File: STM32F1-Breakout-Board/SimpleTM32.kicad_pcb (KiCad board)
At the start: 2 copper layers, 41 x 36 mm, 26 parts, among them J1 USB_B_Micro, J2 Conn_01x15, J3 Conn_01x15, U1 XC6206P332MR, U2 STM32F103C8T6, Y1 8MHz

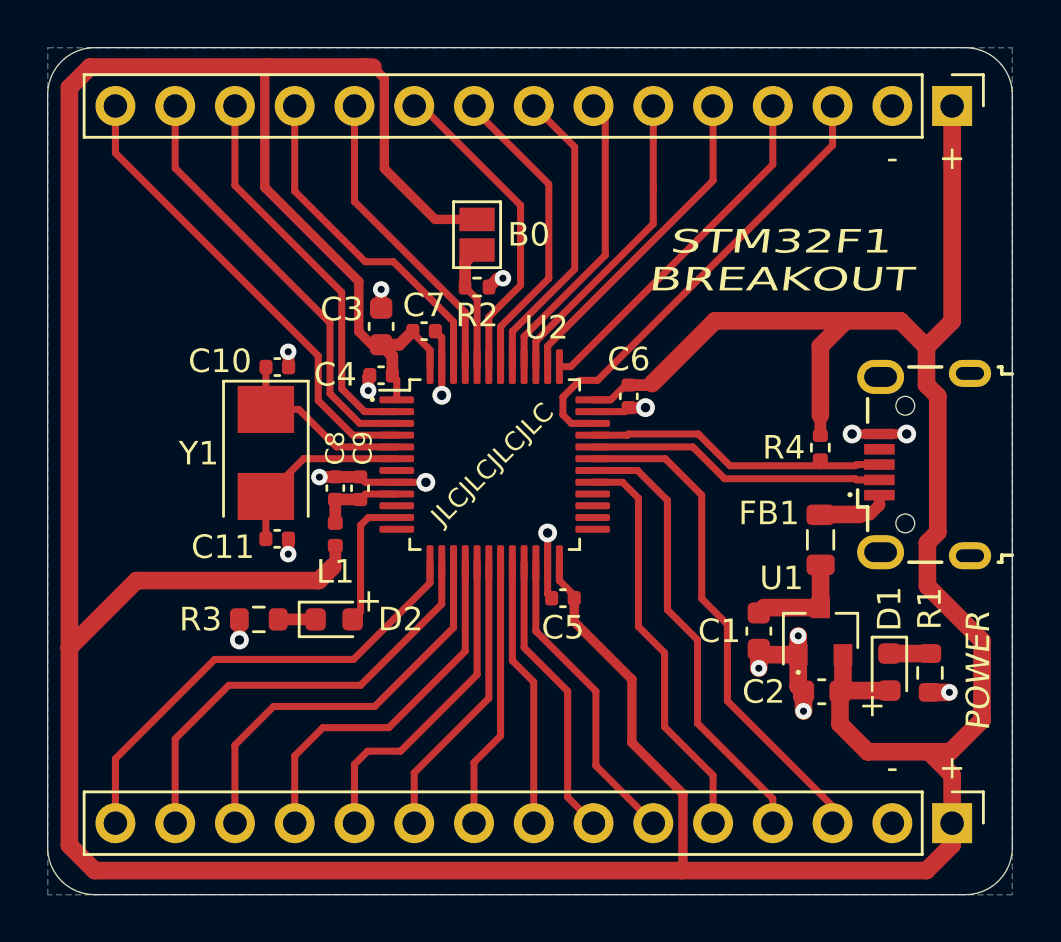
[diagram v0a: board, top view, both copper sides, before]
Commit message: rasp
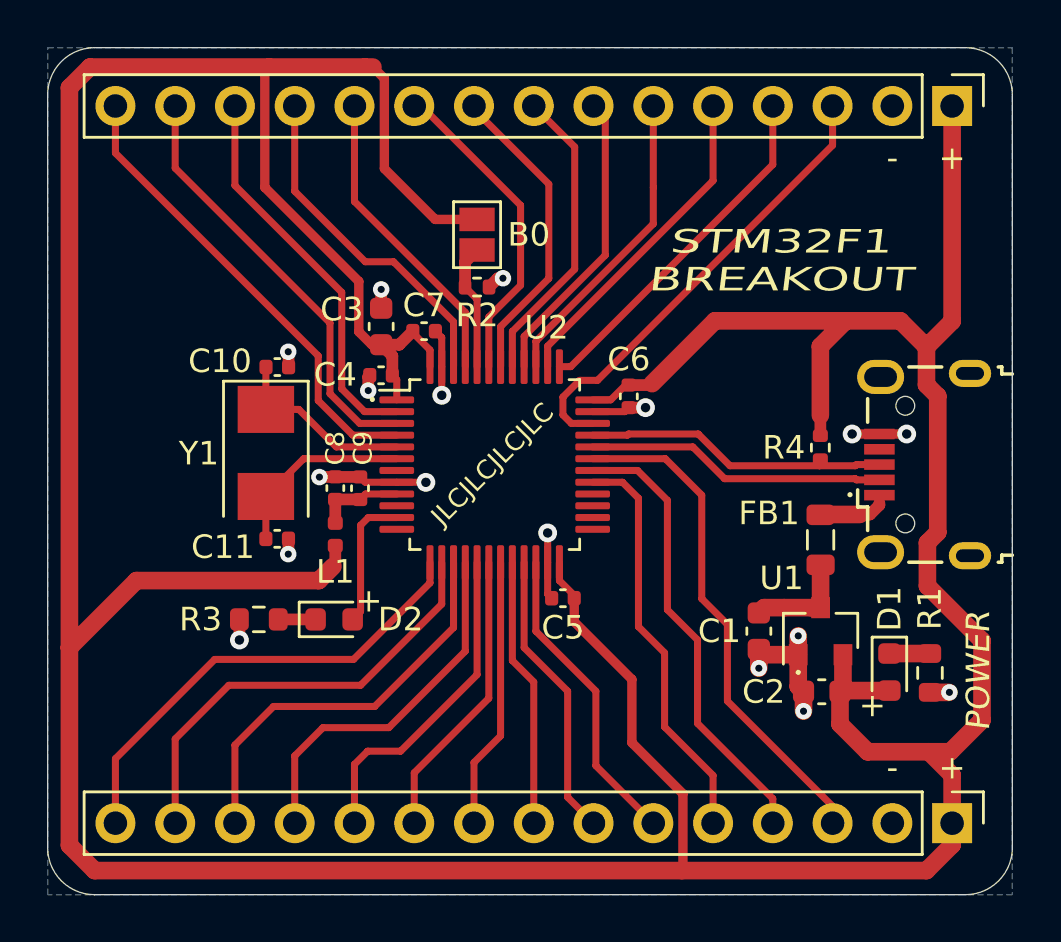
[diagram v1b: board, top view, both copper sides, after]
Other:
- net class Default removed
